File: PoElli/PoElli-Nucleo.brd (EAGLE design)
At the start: 120 parts, among them CN10 NUCLEO-CN10, CN7 NUCLEO-CN7, J3 M022.54MM, J4 M022.54MM, Q3 FDMC2674, Q4 IRFL4310, SW1 A6H2101, SW2 A6H2101, T1 Coilcraft 230NL, T2 FLYBACK750311689, U4 LT3748, U5 TPS2378, U6 ENC424J600, X1 POE-TP-SHIELDED-RJ45-MOLEX-85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, Y1 25 MHz

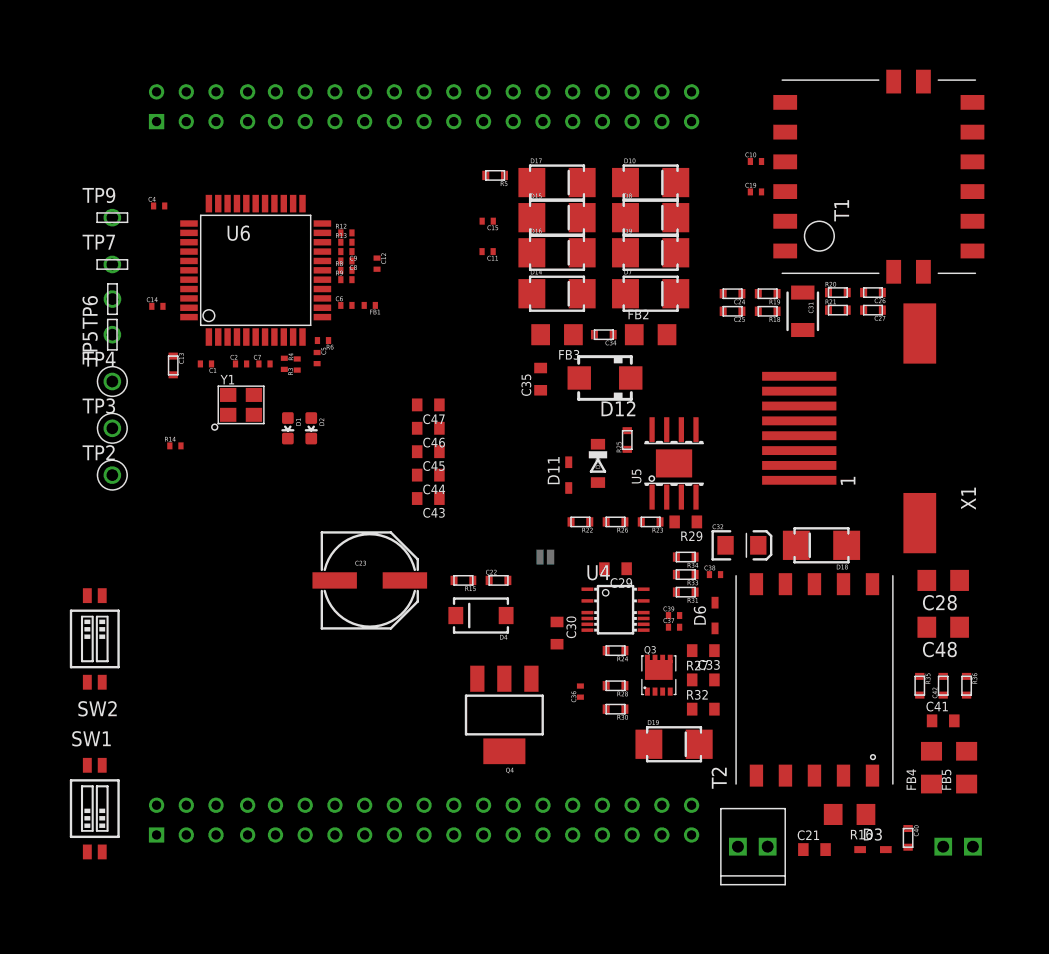
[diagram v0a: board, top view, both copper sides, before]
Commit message: routing draft v0.2, planes & routes in, optimization to be done..
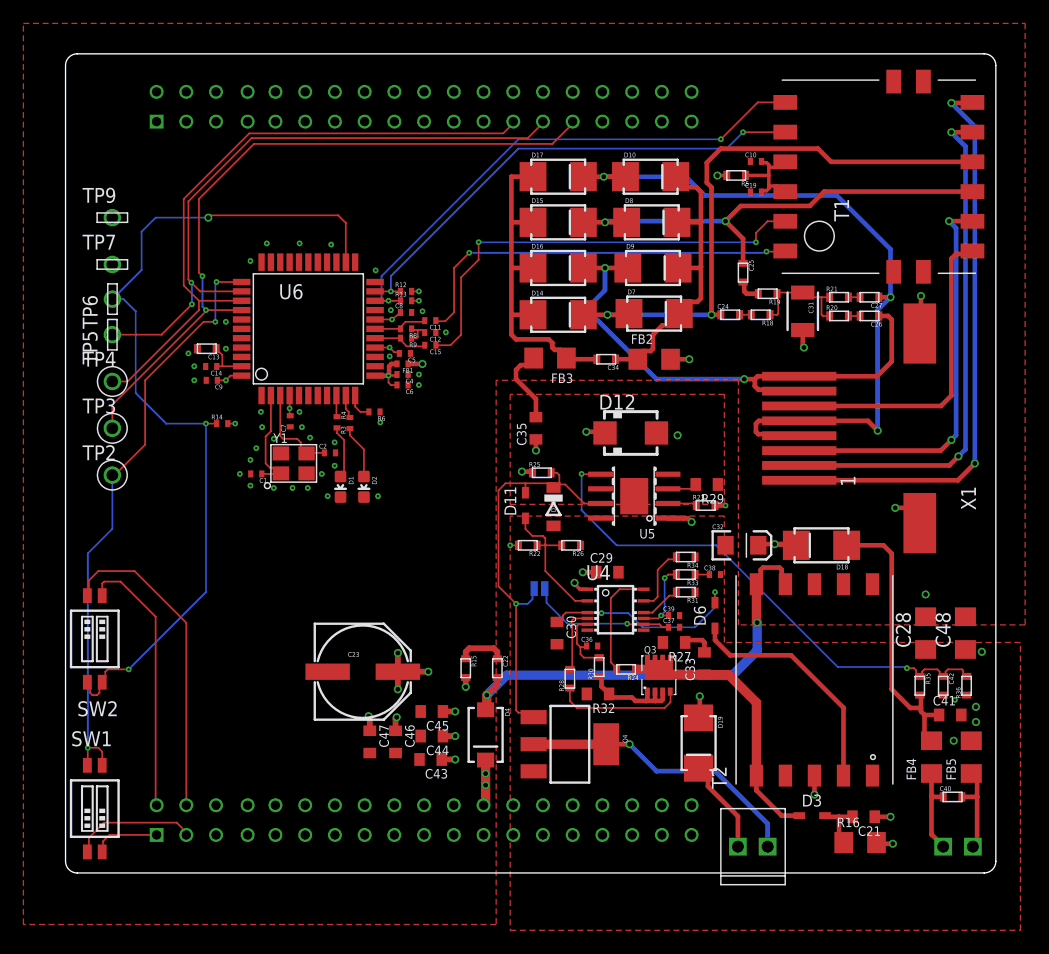
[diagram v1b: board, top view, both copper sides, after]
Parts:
- moved C47 29.2 mm to (26.0, 11.2), turned to 270 degrees
- moved C46 26.9 mm to (28.2, 11.2), turned to 270 degrees
- moved C4 25.3 mm to (28.8, 42.6), turned to 180 degrees
- moved C44 22.3 mm to (31.3, 11.7)
- moved C43 22.3 mm to (31.2, 9.70)
- moved C45 22.2 mm to (31.3, 13.8)
- moved R5 20.6 mm to (57.3, 59.6)
- moved C9 15.9 mm to (12.5, 42.1)
- moved C15 11.7 mm to (31.2, 45.1)
- moved C2 10.7 mm to (22.6, 35.9)
- moved C1 10.3 mm to (16.3, 34.1)
- moved D4 10.2 mm to (35.9, 11.8), turned to 270 degrees
- moved R32 9.09 mm to (45.5, 15.3), turned to 180 degrees
- moved C6 8.32 mm to (28.8, 41.7), turned to 180 degrees
- moved C23 7.82 mm to (25.4, 17.2)
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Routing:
- net ETH_INT: track 0.00 -> 75.6 mm, vias 0 -> 3
- net POE_B+: track 0.00 -> 63.4 mm, vias 0 -> 3
- net ETH_SCK: track 0.00 -> 61.0 mm, vias 0 -> 2
- net ETH_MOSI: track 0.00 -> 54.6 mm
- net ETH_MISO: track 0.00 -> 54.6 mm, vias 0 -> 2
- net ETH_SS: track 0.00 -> 51.3 mm, vias 0 -> 3
- net POE_A+: track 0.00 -> 50.6 mm, vias 0 -> 2
- net N$2: track 0.00 -> 49.0 mm, vias 0 -> 2
- net POE_B-: track 0.00 -> 46.2 mm, vias 0 -> 2
- net TPOUT+: track 0.00 -> 45.4 mm, vias 0 -> 2
- net N$54: track 0.00 -> 45.3 mm, vias 0 -> 2
- net N$1: track 0.00 -> 44.2 mm, vias 0 -> 2
- net TPOUT-: track 0.00 -> 42.3 mm, vias 0 -> 2
- net POE_A-: track 0.00 -> 40.5 mm, vias 0 -> 2
- net UNREG_6V+: track 0.00 -> 39.5 mm, vias 0 -> 2
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- added copper zone on layer 15, net +3V3
- added copper zone on layer 15, net ENC-3V3
- added copper zone on layer 1, net GNDA
- added copper zone on layer 2, net GNDA
- added copper zone on layer 1, net RTN
- added copper zone on layer 2, net RTN
- added copper zone on layer 15, net VDD
- added copper zone on layer 15, net VIN
- added copper zone on layer 1, net VSS
- added copper zone on layer 2, net VSS
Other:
- board outline added: 79.5 x 70 mm
